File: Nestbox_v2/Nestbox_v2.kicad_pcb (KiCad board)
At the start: 2 copper layers, 85 x 60 mm, 125 parts, among them CON301 Micro_SD_Card, J201 BATT_CONN_01X02, J401 LB_DETECT_CONN_01X04, J402 CONN_01X05, J501 CONN_01X01, J502 CONN_01X06, J601 LOAD_CELL_CONN_01X04, J701 RFID_CONN_01X05, P301 RX/TX, P302 TST/RST, P303 DEBUG_3V3, Q201 Q_PMOS_DGS, Q301 NTR3A052PZT1G, Q501 NTR3A052PZT1G, Q601 DMG2301L-7 -- Replace by 0R, Q602 DMG3402L DNP, Q603 DMG2301L-7 DNP, Q604 DMG3402L DNP, Q701 Q_NMOS_GSD, SW301 SMD-BUTTON_2P-3.0X2.5X1.2+0.4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, U201 TPS62745, U202 LTC3534, U203 LP5907, U301 MSP430FR5969, U501 ESP-12S, U601 ADS1220, Y301 Crystal

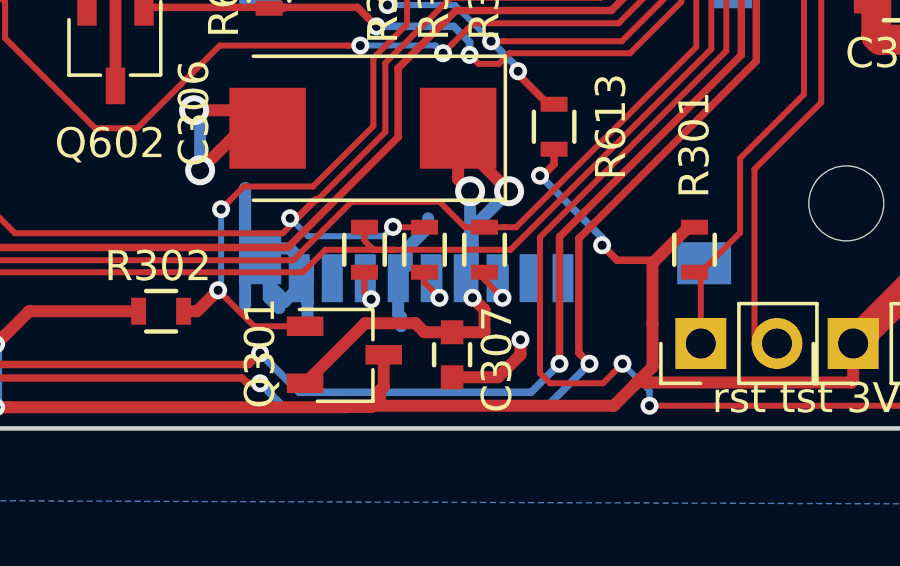
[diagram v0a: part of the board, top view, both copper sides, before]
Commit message: various annotations and changes
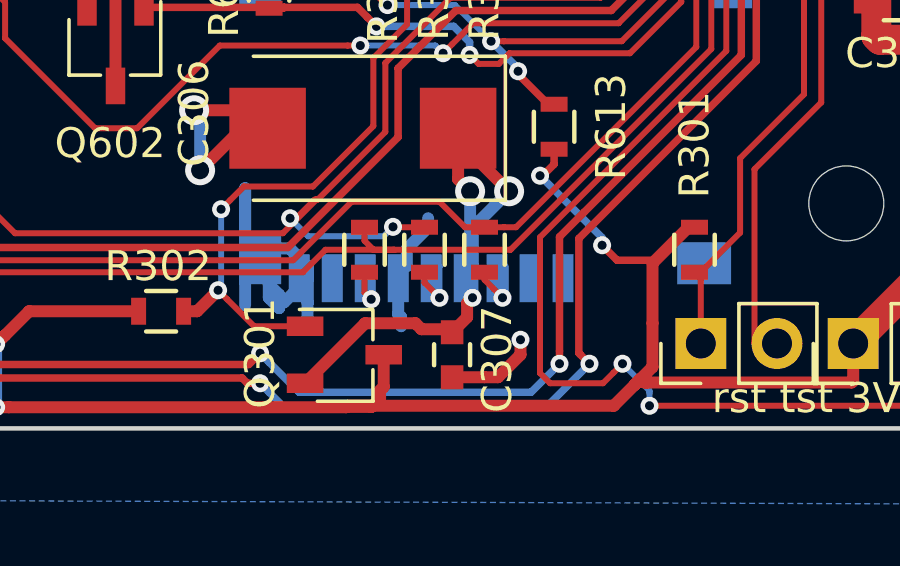
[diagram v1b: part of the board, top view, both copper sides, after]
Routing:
- net Net-(C306-Pad1): track 21.0 -> 19.0 mm
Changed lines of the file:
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@@
   (general
     (links 277)
-    (no_connects 0)
+    (no_connects 1)
     (area -80.29 -82.95 95.35 8.700001)
     (thickness 1.6)
     (drawings 64)
-    (tracks 1751)
+    (tracks 1752)
     (zones 0)
     (modules 125)
@@
   (segment (start 51.975 -18.75) (end 54.5007 -18.75) (width 0.2) (layer F.Cu) (net 7))
   (segment (start 54.5007 -18.75) (end 55 -18.2507) (width 0.2) (layer F.Cu) (net 7))
+  (segment (start 40.71 -0.805) (end 41.11 -1.205) (width 0.4) (layer F.Cu) (net 8))
+  (segment (start 41.11 -1.205) (end 41.11 -1.675) (width 0.4) (layer F.Cu) (net 8))
+  (segment (start 41.11 -1.675) (end 41.29 -1.855) (width 0.4) (layer F.Cu) (net 8))
+  (segment (start 40.61 -0.705) (end 40.71 -0.805) (width 0.2) (layer F.Cu) (net 8))
+  (segment (start 35.71 0.995) (end 37.71 -1.005) (width 0.4) (layer F.Cu) (net 8))
+  (segment (start 37.71 -1.005) (end 39.39 -1.005) (width 0.4) (layer F.Cu) (net 8))
+  (segment (start 39.39 -1.005) (end 39.59 -0.805) (width 0.4) (layer F.Cu) (net 8))
+  (segment (start 39.59 -0.805) (end 40.71 -0.805) (width 0.4) (layer F.Cu) (net 8))
   (segment (start 42.51 -5.405) (end 41.29958 -4.19458) (width 0.4) (layer B.Cu) (net 8))
   (segment (start 41.29958 -4.19458) (end 41.29958 -2.90096) (width 0.4) (layer B.Cu) (net 8))
@@
   (segment (start 40.81 -5.805) (end 41.21 -5.405) (width 0.4) (layer F.Cu) (net 8))
   (via (at 41.21 -5.405) (size 1) (drill 0.6) (layers F.Cu B.Cu) (net 8))
-  (segment (start 40.61 -0.705) (end 41.69 -0.705) (width 0.2) (layer F.Cu) (net 8))
-  (segment (start 35.71 0.995) (end 37.71 -1.005) (width 0.4) (layer F.Cu) (net 8))
-  (segment (start 37.71 -1.005) (end 39.39 -1.005) (width 0.4) (layer F.Cu) (net 8))
-  (segment (start 39.39 -1.005) (end 39.69 -0.705) (width 0.4) (layer F.Cu) (net 8))
   (segment (start 41.29 -1.855) (end 41.29 -2.89138) (width 0.4) (layer B.Cu) (net 8))
   (segment (start 41.29 -2.89138) (end 41.29958 -2.90096) (width 0.4) (layer B.Cu) (net 8))
-  (segment (start 41.69 -0.705) (end 41.69 -1.455) (width 0.4) (layer F.Cu) (net 8))
-  (segment (start 41.69 -1.455) (end 41.29 -1.855) (width 0.4) (layer F.Cu) (net 8))
   (via (at 41.29 -1.855) (size 0.6) (drill 0.3) (layers F.Cu B.Cu) (net 8))
-  (segment (start 39.69 -0.705) (end 41.69 -0.705) (width 0.4) (layer F.Cu) (net 8))
   (segment (start 69.75 -31.75) (end 71.5 -31.75) (width 0.2) (layer F.Cu) (net 9))
   (segment (start 23.5 -28.145) (end 23.5 -27.52) (width 0.4) (layer F.Cu) (net 10))
